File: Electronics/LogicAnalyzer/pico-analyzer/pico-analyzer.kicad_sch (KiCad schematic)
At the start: 12 parts, among them J1 Channels 0-5, J2 Channels 6-11, J3 Channels 12-17, J4 Channels 18-23, J5 USB_C_Receptacle_USB2.0_16P, SW1 SW_DP3T, U7 RP2040_Stamp

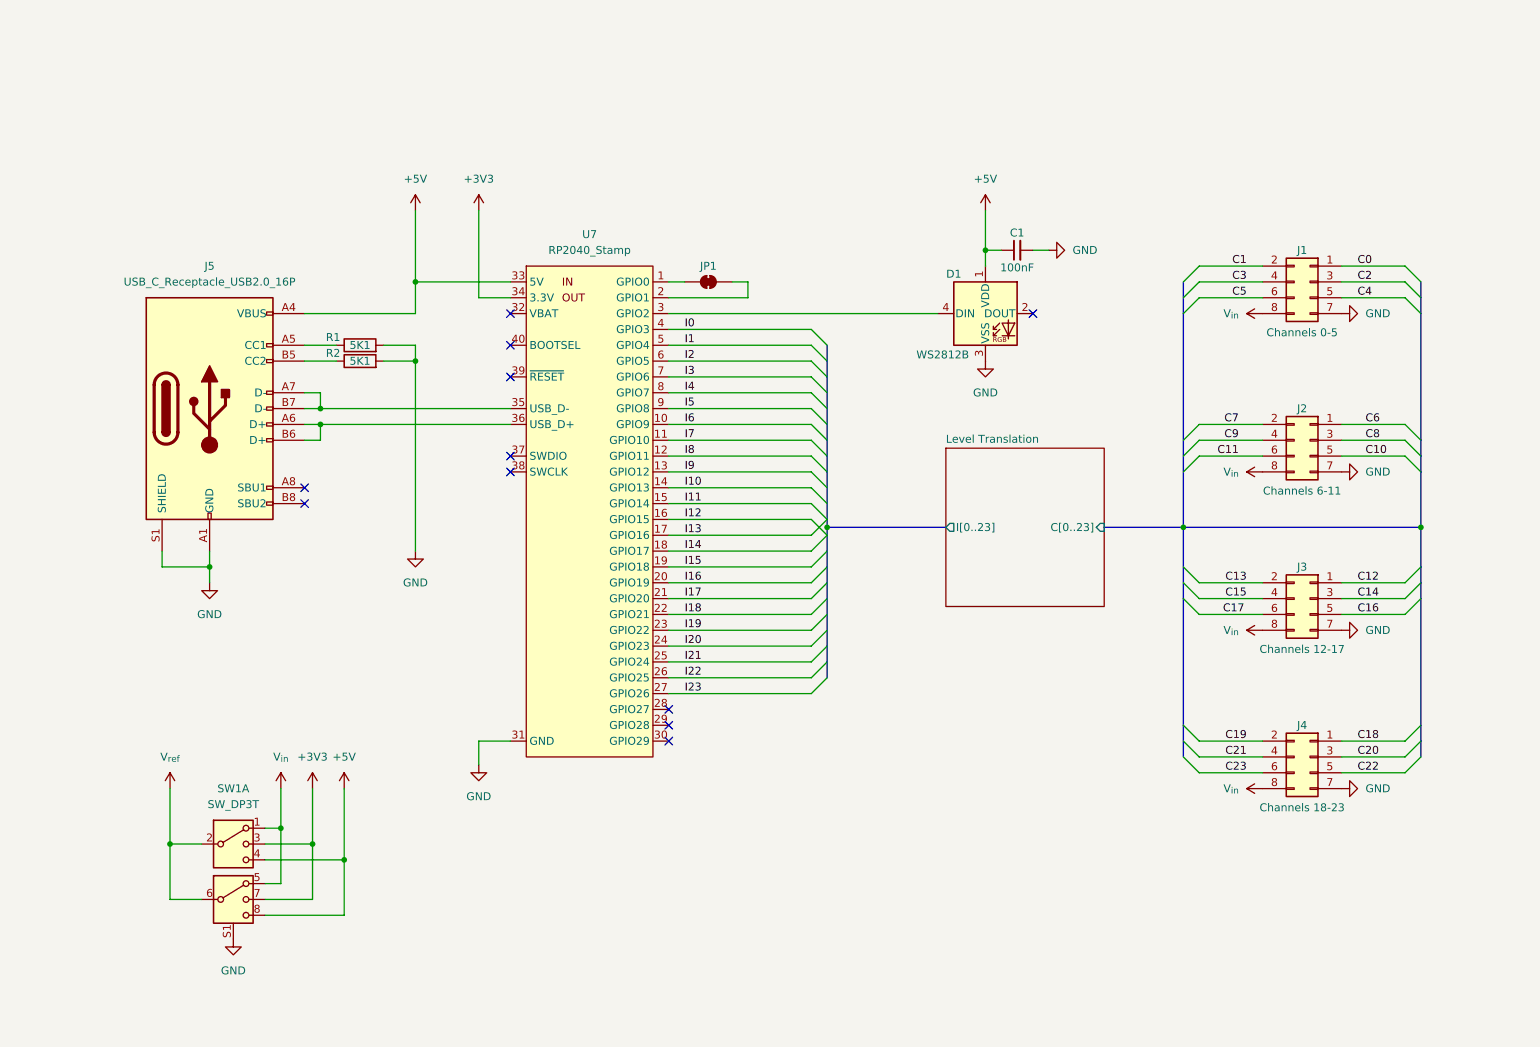
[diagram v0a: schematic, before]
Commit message: Working on pico-analyzer v2
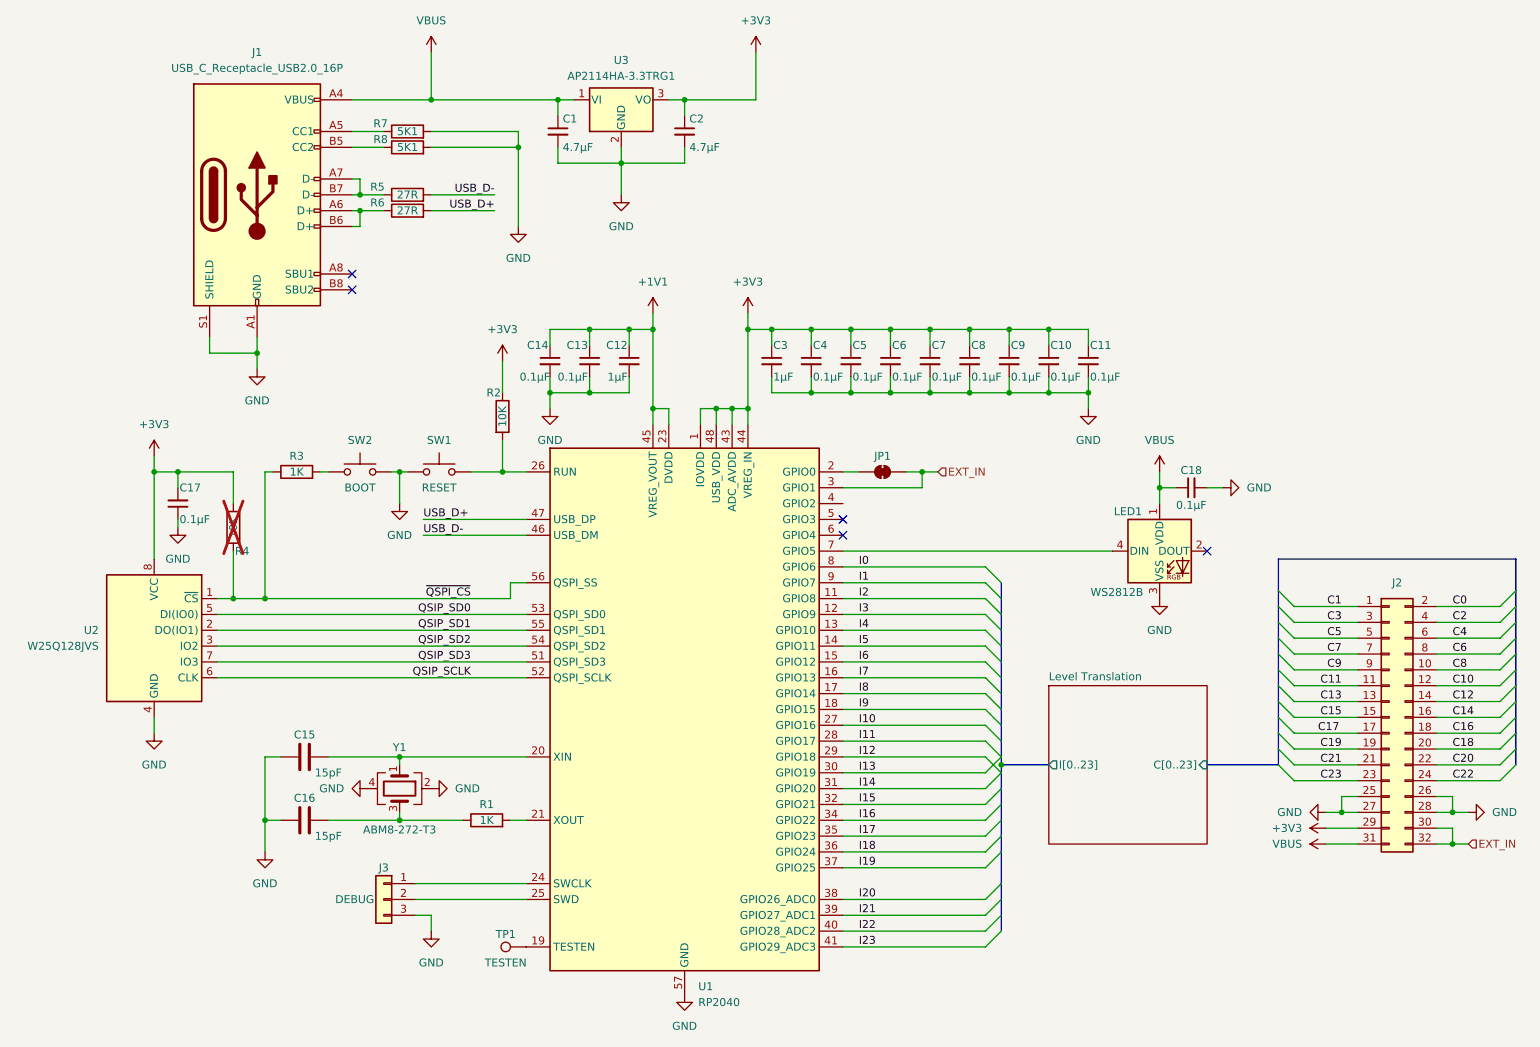
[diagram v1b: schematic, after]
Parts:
- removed J1: Channels 0-5, pico-analyzer:PinHeader_2x04_P2.54mm_Horizontal, symbol Connector_Generic:Conn_02x04_Odd_Even
- removed J2: Channels 6-11, pico-analyzer:PinHeader_2x04_P2.54mm_Horizontal, symbol Connector_Generic:Conn_02x04_Odd_Even
- removed J3: Channels 12-17, pico-analyzer:PinHeader_2x04_P2.54mm_Horizontal, symbol Connector_Generic:Conn_02x04_Odd_Even
- removed J4: Channels 18-23, pico-analyzer:PinHeader_2x04_P2.54mm_Horizontal, symbol Connector_Generic:Conn_02x04_Odd_Even
- removed SW1: SW_DP3T, pico-analyzer:EG2315A, symbol pico-analyzer:SW_DP3T
- removed U7: RP2040_Stamp, pico-analyzer:RP2xxx_Stamp_SMD, symbol pico-analyzer:RP2040_Stamp
- added C1, C2: 4.7µF, Capacitor_SMD:C_0402_1005Metric, symbol Device:C_Small
- added C10, C11, C13, C14, C17, C4, C5, C6, C7, C8, C9: 0.1µF, Capacitor_SMD:C_0402_1005Metric, symbol Device:C_Small
- added C12, C3: 1µF, Capacitor_SMD:C_0402_1005Metric, symbol Device:C_Small
- added C15, C16: 15pF, Capacitor_SMD:C_0402_1005Metric, symbol Device:C
- added J2: Conn_02x16_Odd_Even, Connector_PinHeader_2.54mm:PinHeader_2x16_P2.54mm_Horizontal, symbol Connector_Generic:Conn_02x16_Odd_Even
- added J3: DEBUG, Connector_PinHeader_2.54mm:PinHeader_1x03_P2.54mm_Vertical, symbol Connector_Generic:Conn_01x03
- added R1, R3: 1K, Resistor_SMD:R_0402_1005Metric, symbol Device:R
- added R2, R4: 10K, Resistor_SMD:R_0402_1005Metric, symbol Device:R
- added R5, R6: 27R, Resistor_SMD:R_0402_1005Metric, symbol Device:R
- added SW1: RESET, UPL-Switches:Button_Push_SPST_C&K_PTS647Sx38SMTR2LFS, symbol Switch:SW_Push
- added SW2: BOOT, UPL-Switches:Button_Push_SPST_C&K_PTS647Sx38SMTR2LFS, symbol Switch:SW_Push
- added TP1: TESTEN, TestPoint:TestPoint_Pad_D2.0mm, symbol Connector:TestPoint
- added U1: RP2040, Package_DFN_QFN:QFN-56-1EP_7x7mm_P0.4mm_EP3.2x3.2mm, symbol MCU_RaspberryPi:RP2040
- added U2: W25Q128JVS, Package_SO:SOIC-8_5.23x5.23mm_P1.27mm, symbol Memory_Flash:W25Q128JVS
- added U3: AP2114HA-3.3TRG1, Package_TO_SOT_SMD:SOT-223-3_TabPin2, symbol Regulator_Linear:SPX2920M3-3.3_SOT223
- added Y1: ABM8-272-T3, Crystal:Crystal_SMD_Abracon_ABM8G-4Pin_3.2x2.5mm, symbol Device:Crystal_GND24
- C18: renamed from C1; value 100nF -> 0.1µF; footprint Capacitor_SMD:C_0603_1608Metric -> Capacitor_SMD:C_0402_1005Metric
- R7: renamed from R1; footprint Resistor_SMD:R_0603_1608Metric -> Resistor_SMD:R_0402_1005Metric
- R8: renamed from R2; footprint Resistor_SMD:R_0603_1608Metric -> Resistor_SMD:R_0402_1005Metric
- renumbered J5 to J1, D1 to LED1
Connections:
- net +3V3: now also C10.1, C11.1, C17.2, C2.1, C3.1, C4.1, C5.1, C6.1, C7.1, C8.1, C9.1, J2.29 (Pin_29), R2.1, R4.1, U1.1 (IOVDD), U1.10 (IOVDD), U1.22 (IOVDD), U1.33 (IOVDD), U1.42 (IOVDD), U1.43 (ADC_AVDD), U1.44 (VREG_IN), U1.48 (USB_VDD), U1.49 (IOVDD), U2.8 (VCC), U3.3 (VO)
- net C0: now also J2.2 (Pin_2)
- net C1: now also J2.1 (Pin_1)
- net C10: now also J2.12 (Pin_12)
- net C11: now also J2.11 (Pin_11)
- net C12: now also J2.14 (Pin_14)
- net C13: now also J2.13 (Pin_13)
- net C14: now also J2.16 (Pin_16)
- net C15: now also J2.15 (Pin_15)
- net C16: now also J2.18 (Pin_18)
- net C17: now also J2.17 (Pin_17)
- net C18: now also J2.20 (Pin_20)
- net C19: now also J2.19 (Pin_19)
- net C2: now also J2.4 (Pin_4)
- net C20: now also J2.22 (Pin_22)
- net C21: now also J2.21 (Pin_21)
- net C22: now also J2.24 (Pin_24)
- net C23: now also J2.23 (Pin_23)
- net C3: now also J2.3 (Pin_3)
- net C4: now also J2.6 (Pin_6)
- net C5: now also J2.5 (Pin_5)
- net C6: now also J2.8 (Pin_8)
- net C7: now also J2.7 (Pin_7)
- net C8: now also J2.10 (Pin_10)
- net C9: now also J2.9 (Pin_9)
- net GND: now also C1.2, C10.2, C11.2, C12.2, C13.2, C14.2, C15.1, C16.1, C17.1, C2.2, C3.2, C4.2, C5.2, C6.2, C7.2, C8.2, C9.2, J2.25 (Pin_25), J2.26 (Pin_26), J2.27 (Pin_27), J2.28 (Pin_28), J3.3 (Pin_3), SW1.1, SW2.2, U1.57 (GND), U2.4 (GND), U3.2 (GND), Y1.2, Y1.4
- net I0: now also U1.8 (GPIO6)
- net I1: now also U1.9 (GPIO7)
- net I10: now also U1.27 (GPIO16)
- net I11: now also U1.28 (GPIO17)
- net I12: now also U1.29 (GPIO18)
- net I13: now also U1.30 (GPIO19)
- net I14: now also U1.31 (GPIO20)
- net I15: now also U1.32 (GPIO21)
- net I16: now also U1.34 (GPIO22)
- net I17: now also U1.35 (GPIO23)
- net I18: now also U1.36 (GPIO24)
- net I19: now also U1.37 (GPIO25)
- net I2: now also U1.11 (GPIO8)
- net I20: now also U1.38 (GPIO26_ADC0)
- net I21: now also U1.39 (GPIO27_ADC1)
- net I22: now also U1.40 (GPIO28_ADC2)
- net I23: now also U1.41 (GPIO29_ADC3)
- net I3: now also U1.12 (GPIO9)
- net I4: now also U1.13 (GPIO10)
- net I5: now also U1.14 (GPIO11)
- net I6: now also U1.15 (GPIO12)
- net I7: now also U1.16 (GPIO13)
- net I8: now also U1.17 (GPIO14)
- net I9: now also U1.18 (GPIO15)
- net at JP1.1 (A): now also U1.2 (GPIO0)
- net EXT_IN: now reaches JP1.2 (B)
- net EXT_IN: now also J2.30 (Pin_30), J2.32 (Pin_32), U1.3 (GPIO1)
- net at LED1.4 (DIN): now also U1.7 (GPIO5)
- net at J1.A7 (D-), J1.B7 (D-): now also R5.1
- net at J1.A6 (D+), J1.B6 (D+): now also R6.1
- net +5V renamed VBUS
- net VBUS: now also C1.1, J2.31 (Pin_31), U3.1 (VI)
- new net: C16.2, R1.1, Y1.3
- new net: R1.2, U1.21 (XOUT)
- new net: R2.2, SW1.2, U1.26 (RUN)
- new net: R3.2, SW2.1
- new net: C15.2, U1.20 (XIN), Y1.1
- new net: J3.1 (Pin_1), U1.24 (SWCLK)
- new net: J3.2 (Pin_2), U1.25 (SWD)
- new net: TP1.1, U1.19 (TESTEN)
- new net +1V1: C12.1, C13.1, C14.1, U1.23 (DVDD), U1.45 (VREG_VOUT), U1.50 (DVDD)
- new net QSIP_SCLK: U1.52 (QSPI_SCLK), U2.6 (CLK)
- new net QSIP_SD0: U1.53 (QSPI_SD0), U2.5 (DI(IO0))
- new net QSIP_SD1: U1.55 (QSPI_SD1), U2.2 (DO(IO1))
- new net QSIP_SD2: U1.54 (QSPI_SD2), U2.3 (IO2)
- new net QSIP_SD3: U1.51 (QSPI_SD3), U2.7 (IO3)
- new net USB_D+: R6.2, U1.47 (USB_DP)
- new net USB_D-: R5.2, U1.46 (USB_DM)
- new net ~{QSPI_CS}: R3.1, R4.2, U1.56 (QSPI_SS), U2.1 (~{CS})
- no-connect marks 11 -> 5
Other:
- moved on the sheet: C18, J1, JP1, LED1, R7, R8
